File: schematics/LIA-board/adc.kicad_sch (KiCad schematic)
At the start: 1 part, among them U14 ADS1220xPW

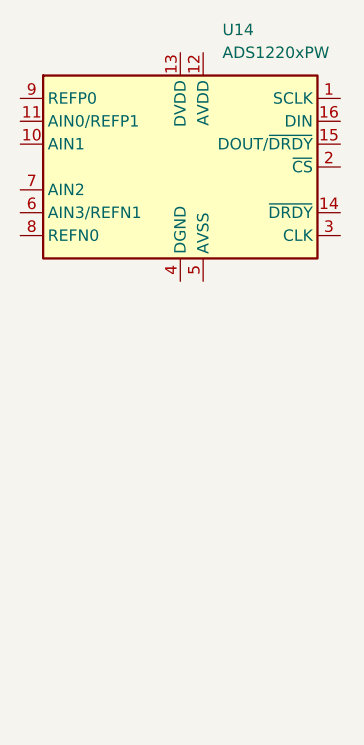
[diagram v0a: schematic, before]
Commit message: all current changes
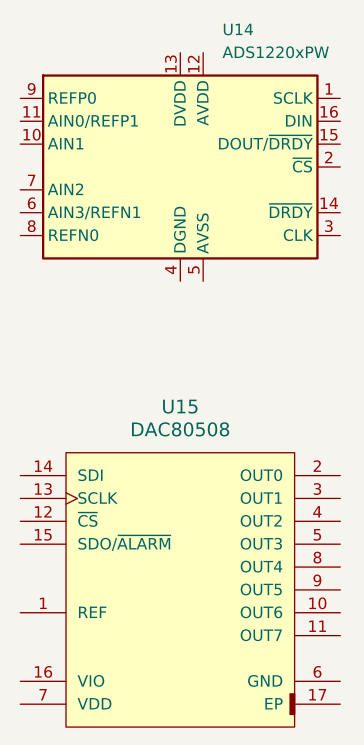
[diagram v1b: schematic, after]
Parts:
- added U15: DAC80508, Package_SON:Texas_DRX_WSON-10_2.5x2.5mm_P0.5mm, symbol CERN:DAC80508ZRTE
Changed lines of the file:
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@@
+		)
+	)
+	(symbol
+		(lib_id "CERN:DAC80508ZRTE")
+		(at 137.16 119.38 0)
+		(unit 1)
+		(body_style 1)
+		(exclude_from_sim no)
+		(in_bom yes)
+		(on_board yes)
+		(in_pos_files yes)
+		(dnp no)
+		(fields_autoplaced yes)
+		(property "Reference" "U15"
+			(at 149.86 114.3 0)
+			(show_name no)
+			(do_not_autoplace no)
+			(effects
+				(font
+					(size 1.524 1.524)
+				)
+			)
+		)
+		(property "Value" "DAC80508"
+			(at 149.86 116.84 0)
+			(show_name no)
+			(do_not_autoplace no)
+			(effects
+				(font
+					(size 1.524 1.524)
+				)
+			)
+		)
+		(property "Footprint" "Package_SON:Texas_DRX_WSON-10_2.5x2.5mm_P0.5mm"
+			(at 137.16 119.38 0)
+			(hide yes)
+			(show_name no)
+			(do_not_autoplace no)
+			(effects
+				(font
+					(size 1.27 1.27)
+				)
+			)
+		)
+		(property "Datasheet" ""
+			(at 137.16 119.38 0)
+			(hide yes)
+			(show_name no)
+			(do_not_autoplace no)
+			(effects
+				(font
+					(size 1.27 1.27)
+				)
+			)
+		)
+		(property "Description" "Octal, 16-Bit, SPI, Voltage Output DAC With Internal Reference"
+			(at 137.16 119.38 0)
+			(hide yes)
+			(show_name no)
+			(do_not_autoplace no)
+			(effects
+				(font
+					(size 1.27 1.27)
+				)
+			)
+		)
+		(pin "9"
+		)
+		(pin "10"
+		)
+		(pin "11"
+		)
+		(pin "12"
+		)
+		(pin "13"
+		)
+		(pin "14"
+		)
+		(pin "15"
+		)
+		(pin "16"
+		)
+		(pin "1"
+		)
+		(pin "4"
+		)
+		(pin "5"
+		)
+		(pin "3"
+		)
+		(pin "2"
+		)
+		(pin "17"
+		)
+		(pin "6"
+		)
+		(pin "7"
+		)
+		(pin "8"
+		)
+		(instances
+			(project "GMOS-LIA"
+				(path "/87b3d1ed-39bd-4cff-a405-e580c48ff0ef/c2b448c7-1606-40e4-b2d6-d927d0381aee"
+					(reference "U15")
+					(unit 1)
+				)
+			)
 		)
 	)
